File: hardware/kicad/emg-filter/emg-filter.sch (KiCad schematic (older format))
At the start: 14 parts

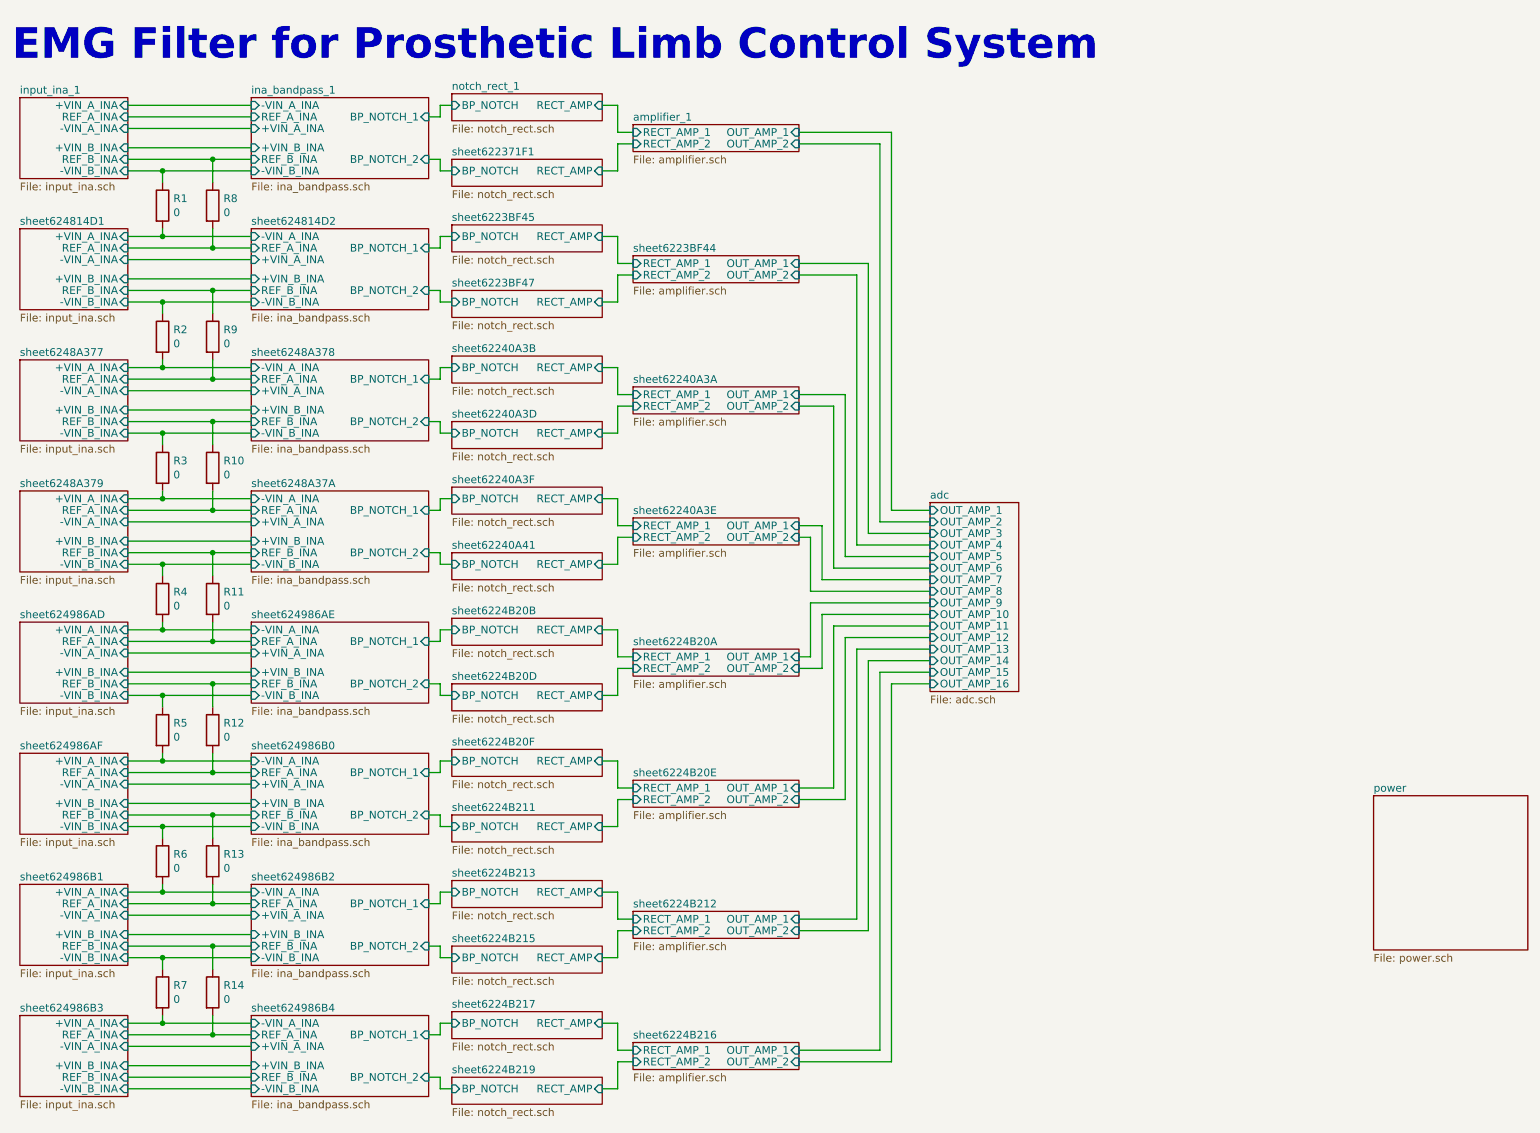
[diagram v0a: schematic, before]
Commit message: update
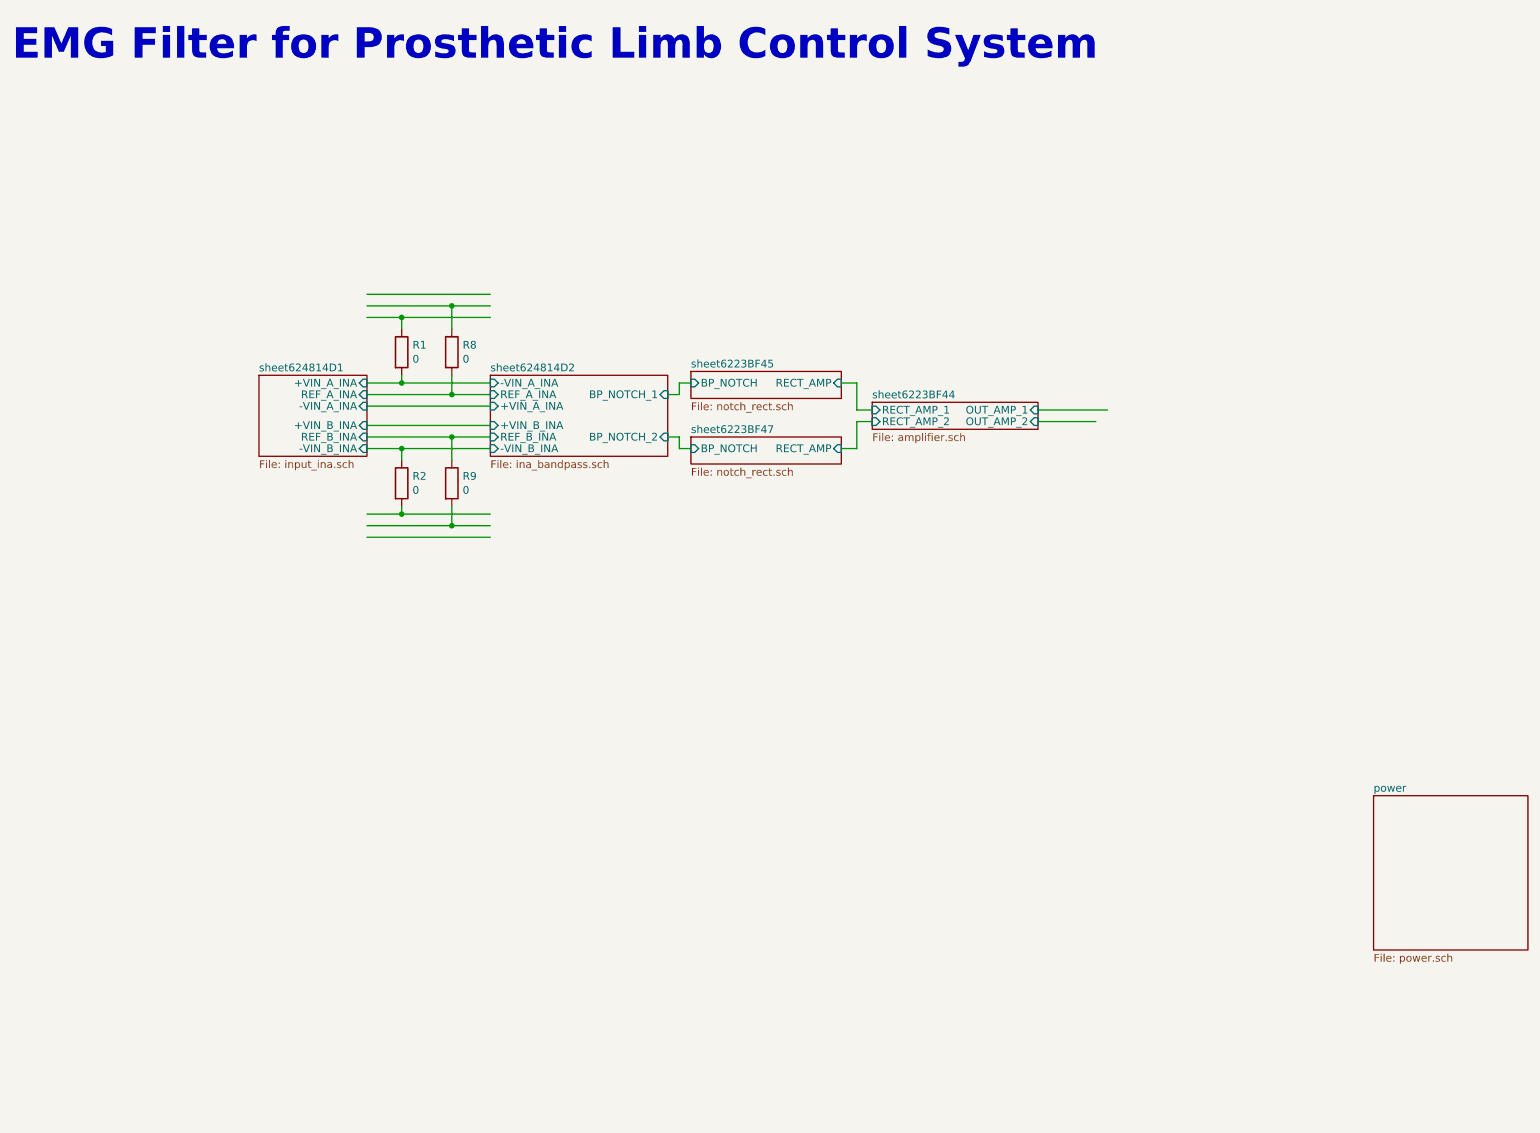
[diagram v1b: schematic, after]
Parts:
- removed R10, R11, R12, R13, R14, R3, R4, R5, R6, R7: 0, Resistor_SMD:R_0805_2012Metric, symbol Device:R
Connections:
- wire segments 248 -> 42
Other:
- moved on the sheet: R1, R2, R8, R9

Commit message: update
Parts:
- added J? (x3): Conn_01x02, emg-filter:EMG_CONN_01x02, symbol Connector_Generic:Conn_01x02
- added J? (x2): Conn_01x05, symbol Connector_Generic:Conn_01x05
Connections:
- wire segments 42 -> 49
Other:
- moved on the sheet: R1, R2, R8, R9
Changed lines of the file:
@@
 Text Notes 500  825  0    197  ~ 39
 EMG Filter for Prosthetic Limb Control System
-Wire Wire Line
-	7150 3075 7600 3075
-Wire Wire Line
-	7525 3150 7150 3150
 $Sheet
 S 4900 3250 975  175
@@
 $EndSheet
 Wire Wire Line
-	2800 2400 3350 2400
-Wire Wire Line
-	2800 2325 3600 2325
-$Sheet
-S 2100 2850 700  525
+	4650 1375 5200 1375
+Wire Wire Line
+	4650 1300 5450 1300
+$Sheet
+S 1950 2850 850  525
 U 624814DA
 F0 "sheet624814D1" 50
@@
 	4825 3325 4900 3325
 Wire Wire Line
-	2800 3325 3025 3325
-Wire Wire Line
-	2800 3250 3350 3250
-Wire Wire Line
 	2800 3175 3600 3175
 Wire Wire Line
 	2800 3050 3600 3050
 Wire Wire Line
-	2800 2975 3350 2975
-Wire Wire Line
-	2800 2900 3025 2900
-Wire Wire Line
-	2800 3900 3600 3900
-Wire Wire Line
-	2800 3825 3350 3825
-Wire Wire Line
-	2800 3750 3025 3750
+	2800 2975 3250 2975
 $Comp
 L Device:R R?
 U 1 1 624AA066
-P 3025 2700
+P 4875 1675
 AR Path="/61C386B1/624AA066" Ref="R?"  Part="1"
 AR Path="/61C389A8/624AA066" Ref="R?"  Part="1"
@@
 AR Path="/62498716/624AA066" Ref="R?"  Part="1"
 AR Path="/624AA066" Ref="R1"  Part="1"
-F 0 "R1" H 3095 2746 50  0000 L CNN
-F 1 "0" H 3095 2655 50  0000 L CNN
-F 2 "Resistor_SMD:R_0805_2012Metric" V 2955 2700 50  0001 C CNN
-F 3 "~" H 3025 2700 50  0001 C CNN
-	1    3025 2700
+F 0 "R1" H 4945 1721 50  0000 L CNN
+F 1 "0" H 4945 1630 50  0000 L CNN
+F 2 "Resistor_SMD:R_0805_2012Metric" V 4805 1675 50  0001 C CNN
+F 3 "~" H 4875 1675 50  0001 C CNN
+	1    4875 1675
 	1    0    0    -1
 $EndComp
@@
 L Device:R R?
 U 1 1 624BBA9E
-P 3350 2700
+P 5200 1675
 AR Path="/61C386B1/624BBA9E" Ref="R?"  Part="1"
 AR Path="/61C389A8/624BBA9E" Ref="R?"  Part="1"
@@
 AR Path="/62498716/624BBA9E" Ref="R?"  Part="1"
 AR Path="/624BBA9E" Ref="R8"  Part="1"
-F 0 "R8" H 3420 2746 50  0000 L CNN
-F 1 "0" H 3420 2655 50  0000 L CNN
-F 2 "Resistor_SMD:R_0805_2012Metric" V 3280 2700 50  0001 C CNN
-F 3 "~" H 3350 2700 50  0001 C CNN
-	1    3350 2700
+F 0 "R8" H 5270 1721 50  0000 L CNN
+F 1 "0" H 5270 1630 50  0000 L CNN
+F 2 "Resistor_SMD:R_0805_2012Metric" V 5130 1675 50  0001 C CNN
+F 3 "~" H 5200 1675 50  0001 C CNN
+	1    5200 1675
 	1    0    0    -1
 $EndComp
 Wire Wire Line
-	2800 2475 3025 2475
-Wire Wire Line
-	3025 2475 3025 2550
-Connection ~ 3025 2475
-Wire Wire Line
-	3025 2475 3600 2475
-Wire Wire Line
-	3350 2400 3350 2550
-Connection ~ 3350 2400
-Wire Wire Line
-	3350 2400 3600 2400
-Wire Wire Line
-	3025 2850 3025 2900
-Connection ~ 3025 2900
-Wire Wire Line
-	3025 2900 3600 2900
-Wire Wire Line
-	3350 2850 3350 2975
-Connection ~ 3350 2975
-Wire Wire Line
-	3350 2975 3600 2975
+	4650 1450 4875 1450
+Wire Wire Line
+	4875 1450 4875 1525
+Connection ~ 4875 1450
+Wire Wire Line
+	4875 1450 5450 1450
+Wire Wire Line
+	5200 1375 5200 1525
+Connection ~ 5200 1375
+Wire Wire Line
+	5200 1375 5450 1375
+$Comp
+L Connector_Generic:Conn_01x02 J?
+U 1 1 61F541EB
+P 3250 2550
+AR Path="/61C386B1/61F541EB" Ref="J?"  Part="1"
+AR Path="/61C389A8/61F541EB" Ref="J?"  Part="1"
+AR Path="/622FC90E/61F541EB" Ref="J?"  Part="1"
+AR Path="/623EBE47/61F541EB" Ref="J?"  Part="1"
+AR Path="/624814DA/61F541EB" Ref="J?"  Part="1"
+AR Path="/6248A382/61F541EB" Ref="J?"  Part="1"
+AR Path="/6248A3A0/61F541EB" Ref="J?"  Part="1"
+AR Path="/624986BC/61F541EB" Ref="J?"  Part="1"
+AR Path="/624986DA/61F541EB" Ref="J?"  Part="1"
+AR Path="/624986F8/61F541EB" Ref="J?"  Part="1"
+AR Path="/62498716/61F541EB" Ref="J?"  Part="1"
+AR Path="/61F541EB" Ref="J?"  Part="1"
+F 0 "J?" H 3775 2550 50  0000 R CNN
+F 1 "Conn_01x02" H 3775 2450 50  0000 R CNN
+F 2 "emg-filter:EMG_CONN_01x02" H 3250 2550 50  0001 C CNN
+F 3 "~" H 3250 2550 50  0001 C CNN
+	1    3250 2550
+	0    1    -1   0
+$EndComp
+Wire Wire Line
+	3250 2750 3250 2975
+Connection ~ 3250 2975
+Wire Wire Line
+	3150 2750 3150 2900
+Connection ~ 3150 2900
+Wire Wire Line
+	3150 2900 3600 2900
+Wire Wire Line
+	2800 2900 3150 2900
+Wire Wire Line
+	3250 2975 3600 2975
+Wire Wire Line
+	2800 3250 3250 3250
+$Comp
+L Connector_Generic:Conn_01x02 J?
+U 1 1 61F5D7D3
+P 3250 3675
+AR Path="/61C386B1/61F5D7D3" Ref="J?"  Part="1"
+AR Path="/61C389A8/61F5D7D3" Ref="J?"  Part="1"
+AR Path="/622FC90E/61F5D7D3" Ref="J?"  Part="1"
+AR Path="/623EBE47/61F5D7D3" Ref="J?"  Part="1"
+AR Path="/624814DA/61F5D7D3" Ref="J?"  Part="1"
+AR Path="/6248A382/61F5D7D3" Ref="J?"  Part="1"
+AR Path="/6248A3A0/61F5D7D3" Ref="J?"  Part="1"
+AR Path="/624986BC/61F5D7D3" Ref="J?"  Part="1"
+AR Path="/624986DA/61F5D7D3" Ref="J?"  Part="1"
+AR Path="/624986F8/61F5D7D3" Ref="J?"  Part="1"
+AR Path="/62498716/61F5D7D3" Ref="J?"  Part="1"
+AR Path="/61F5D7D3" Ref="J?"  Part="1"
+F 0 "J?" H 3775 3675 50  0000 R CNN
+F 1 "Conn_01x02" H 3775 3575 50  0000 R CNN
+F 2 "emg-filter:EMG_CONN_01x02" H 3250 3675 50  0001 C CNN
+F 3 "~" H 3250 3675 50  0001 C CNN
+	1    3250 3675
+	0    1    1    0
+$EndComp
+Wire Wire Line
+	3250 3475 3250 3250
+Connection ~ 3250 3250
+Wire Wire Line
+	3150 3325 3150 3475
+Connection ~ 3150 3325
+Wire Wire Line
+	3150 3325 3600 3325
+Wire Wire Line
+	2800 3325 3150 3325
+Wire Wire Line
+	3250 3250 3600 3250
+$Comp
+L Connector_Generic:Conn_01x05 J?
+U 1 1 61F69EB5
+P 7725 3675
+F 0 "J?" V 7597 3955 50  0000 L CNN
+F 1 "Conn_01x05" V 7688 3955 50  0000 L CNN
+F 2 "" H 7725 3675 50  0001 C CNN
+F 3 "~" H 7725 3675 50  0001 C CNN
+	1    7725 3675
+	0    1    1    0
+$EndComp
+$Comp
+L Connector_Generic:Conn_01x05 J?
+U 1 1 61F6D9FD
+P 7725 2550
+F 0 "J?" V 7689 2830 50  0000 L CNN
+F 1 "Conn_01x05" V 7598 2830 50  0000 L CNN
+F 2 "" H 7725 2550 50  0001 C CNN
+F 3 "~" H 7725 2550 50  0001 C CNN
+	1    7725 2550
+	0    1    -1   0
+$EndComp
+Wire Wire Line
+	7725 2750 7725 3475
+Wire Wire Line
+	7525 2750 7525 3075
+Wire Wire Line
+	7625 3150 7150 3150
+Connection ~ 7625 3150
+Wire Wire Line
+	7625 3150 7625 3475
+Wire Wire Line
+	7625 2750 7625 3150
+Wire Wire Line
+	7525 3075 7150 3075
+Connection ~ 7525 3075
+Wire Wire Line
+	7525 3075 7525 3475
+Wire Wire Line
+	7825 2750 7825 3475
+Wire Wire Line
+	7925 3475 7925 2750
+Wire Wire Line
+	3000 4750 3575 4750
+Wire Wire Line
+	3000 4700 3000 4750
+Wire Wire Line
+	3325 4825 3575 4825
+Wire Wire Line
+	3325 4700 3325 4825
+$Comp
+L Device:R R?
+U 1 1 6274723C
+P 3325 4550
+AR Path="/61C386B1/6274723C" Ref="R?"  Part="1"
+AR Path="/61C389A8/6274723C" Ref="R?"  Part="1"
+AR Path="/622FC90E/6274723C" Ref="R?"  Part="1"
+AR Path="/623EBE47/6274723C" Ref="R?"  Part="1"
+AR Path="/624814DA/6274723C" Ref="R?"  Part="1"
+AR Path="/6248A382/6274723C" Ref="R?"  Part="1"
+AR Path="/6248A3A0/6274723C" Ref="R?"  Part="1"
+AR Path="/624986BC/6274723C" Ref="R?"  Part="1"
+AR Path="/624986DA/6274723C" Ref="R?"  Part="1"
+AR Path="/624986F8/6274723C" Ref="R?"  Part="1"
+AR Path="/62498716/6274723C" Ref="R?"  Part="1"
+AR Path="/6274723C" Ref="R9"  Part="1"
+F 0 "R9" H 3395 4596 50  0000 L CNN
+F 1 "0" H 3395 4505 50  0000 L CNN
+F 2 "Resistor_SMD:R_0805_2012Metric" V 3255 4550 50  0001 C CNN
+F 3 "~" H 3325 4550 50  0001 C CNN
+	1    3325 4550
+	1    0    0    -1
+$EndComp
 $Comp
 L Device:R R?
 U 1 1 62747236
-P 3025 3550
+P 3000 4550
 AR Path="/61C386B1/62747236" Ref="R?"  Part="1"
 AR Path="/61C389A8/62747236" Ref="R?"  Part="1"
@@
 AR Path="/62498716/62747236" Ref="R?"  Part="1"
 AR Path="/62747236" Ref="R2"  Part="1"
-F 0 "R2" H 3095 3596 50  0000 L CNN
-F 1 "0" H 3095 3505 50  0000 L CNN
-F 2 "Resistor_SMD:R_0805_2012Metric" V 2955 3550 50  0001 C CNN
-F 3 "~" H 3025 3550 50  0001 C CNN
-	1    3025 3550
+F 0 "R2" H 3070 4596 50  0000 L CNN
+F 1 "0" H 3070 4505 50  0000 L CNN
+F 2 "Resistor_SMD:R_0805_2012Metric" V 2930 4550 50  0001 C CNN
+F 3 "~" H 3000 4550 50  0001 C CNN
+	1    3000 4550
 	1    0    0    -1
 $EndComp
-$Comp
-L Device:R R?
-U 1 1 6274723C
-P 3350 3550
-AR Path="/61C386B1/6274723C" Ref="R?"  Part="1"
-AR Path="/61C389A8/6274723C" Ref="R?"  Part="1"
-AR Path="/622FC90E/6274723C" Ref="R?"  Part="1"
-AR Path="/623EBE47/6274723C" Ref="R?"  Part="1"
-AR Path="/624814DA/6274723C" Ref="R?"  Part="1"
-AR Path="/6248A382/6274723C" Ref="R?"  Part="1"
-AR Path="/6248A3A0/6274723C" Ref="R?"  Part="1"
-AR Path="/624986BC/6274723C" Ref="R?"  Part="1"
-AR Path="/624986DA/6274723C" Ref="R?"  Part="1"
-AR Path="/624986F8/6274723C" Ref="R?"  Part="1"
-AR Path="/62498716/6274723C" Ref="R?"  Part="1"
-AR Path="/6274723C" Ref="R9"  Part="1"
-F 0 "R9" H 3420 3596 50  0000 L CNN
-F 1 "0" H 3420 3505 50  0000 L CNN
-F 2 "Resistor_SMD:R_0805_2012Metric" V 3280 3550 50  0001 C CNN
-F 3 "~" H 3350 3550 50  0001 C CNN
-	1    3350 3550
-	1    0    0    -1
-$EndComp
-Wire Wire Line
-	3025 3400 3025 3325
-Connection ~ 3025 3325
-Wire Wire Line
-	3025 3325 3600 3325
-Wire Wire Line
-	3350 3400 3350 3250
-Connection ~ 3350 3250
-Wire Wire Line
-	3350 3250 3600 3250
-Wire Wire Line
-	3350 3700 3350 3825
-Connection ~ 3350 3825
-Wire Wire Line
-	3350 3825 3600 3825
-Wire Wire Line
-	3025 3700 3025 3750
-Connection ~ 3025 3750
-Wire Wire Line
-	3025 3750 3600 3750
+Connection ~ 3000 4750
+Wire Wire Line
+	2775 4750 3000 4750
+Connection ~ 3325 4825
+Wire Wire Line
+	2775 4825 3325 4825
+Wire Wire Line
+	2775 4900 3575 4900
+$Comp
+L Connector_Generic:Conn_01x02 J?
+U 1 1 61F7C54C
+P 3150 1600
+AR Path="/61C386B1/61F7C54C" Ref="J?"  Part="1"
+AR Path="/61C389A8/61F7C54C" Ref="J?"  Part="1"
+AR Path="/622FC90E/61F7C54C" Ref="J?"  Part="1"
+AR Path="/623EBE47/61F7C54C" Ref="J?"  Part="1"
+AR Path="/624814DA/61F7C54C" Ref="J?"  Part="1"
+AR Path="/6248A382/61F7C54C" Ref="J?"  Part="1"
+AR Path="/6248A3A0/61F7C54C" Ref="J?"  Part="1"
+AR Path="/624986BC/61F7C54C" Ref="J?"  Part="1"
+AR Path="/624986DA/61F7C54C" Ref="J?"  Part="1"
+AR Path="/624986F8/61F7C54C" Ref="J?"  Part="1"
+AR Path="/62498716/61F7C54C" Ref="J?"  Part="1"
+AR Path="/61F7C54C" Ref="J?"  Part="1"
+F 0 "J?" H 3675 1600 50  0000 R CNN
+F 1 "Conn_01x02" H 3675 1500 50  0000 R CNN
+F 2 "emg-filter:EMG_CONN_01x02" H 3150 1600 50  0001 C CNN
+F 3 "~" H 3150 1600 50  0001 C CNN
+	1    3150 1600
+	0    -1   1    0
+$EndComp
 $EndSCHEMATC
